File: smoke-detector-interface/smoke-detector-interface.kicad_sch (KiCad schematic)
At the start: 28 parts, among them J1 Conn_01x04_Pin, J2 M50-3500542, J3 DE9_Receptacle, J4 61200621621, J5 Conn_01x06_Pin, U1 UA78L10ACLPRE3, U2 AS7805AT, U3 ATtiny13A-P

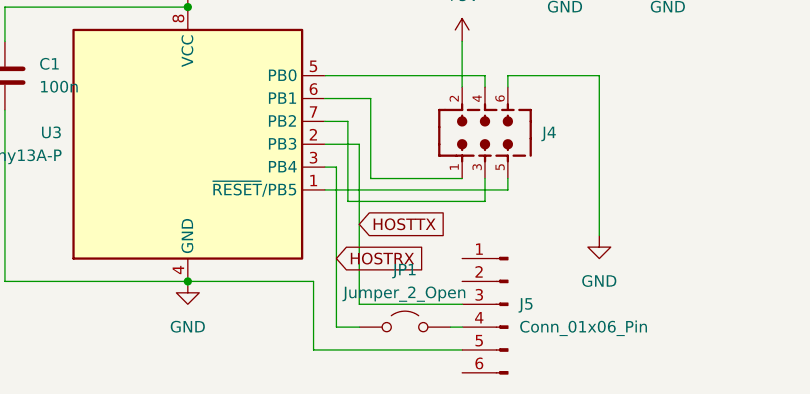
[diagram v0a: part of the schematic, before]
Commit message: WIP
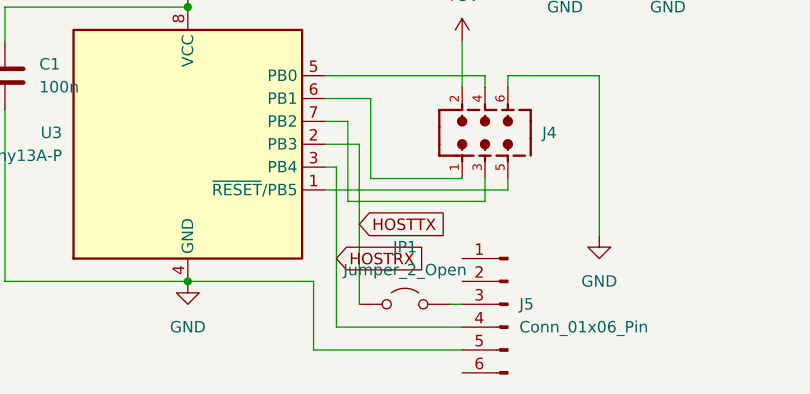
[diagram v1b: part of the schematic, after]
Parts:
- JP1: footprint TestPoint:TestPoint_Bridge_Pitch2.54mm_Drill0.7mm -> Resistor_THT:R_Axial_DIN0204_L3.6mm_D1.6mm_P7.62mm_Horizontal
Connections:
- net HOSTRX: now also J5.4 (Pin_4); no longer JP1.1 (A)
- net HOSTTX: now also JP1.1 (A); no longer J5.3 (Pin_3)
- net at JP1.2 (B): now also J5.3 (Pin_3); no longer J5.4 (Pin_4)
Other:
- moved on the sheet: JP1
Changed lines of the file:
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@@
 	(wire
 		(pts
-			(xy 196.85 143.51) (xy 194.31 143.51)
+			(xy 194.31 143.51) (xy 208.28 143.51)
 		)
 		(stroke
@@
 	(wire
 		(pts
-			(xy 208.28 140.97) (xy 196.85 140.97)
+			(xy 208.28 140.97) (xy 207.01 140.97)
 		)
 		(stroke
@@
 	(wire
 		(pts
-			(xy 208.28 143.51) (xy 207.01 143.51)
-		)
-		(stroke
-			(width 0)
-			(type default)
-		)
-	)
-	(wire
-		(pts
 			(xy 231.14 88.9) (xy 231.14 91.44)
 		)
@@
 	(symbol
 		(lib_id "Jumper:Jumper_2_Open")
-		(at 201.93 143.51 0)
+		(at 201.93 140.97 0)
 		(unit 1)
 		(exclude_from_sim yes)
@@
 		(fields_autoplaced yes)
 		(property "Reference" "JP1"
-			(at 201.93 137.16 0)
+			(at 201.93 134.62 0)
 			(effects
 				(font
@@
 		)
 		(property "Value" "Jumper_2_Open"
-			(at 201.93 139.7 0)
+			(at 201.93 137.16 0)
 			(effects
 				(font
@@
 			)
 		)
-		(property "Footprint" "TestPoint:TestPoint_Bridge_Pitch2.54mm_Drill0.7mm"
-			(at 201.93 143.51 0)
+		(property "Footprint" "Resistor_THT:R_Axial_DIN0204_L3.6mm_D1.6mm_P7.62mm_Horizontal"
+			(at 201.93 140.97 0)
 			(effects
 				(font
@@
 		)
 		(property "Datasheet" "~"
-			(at 201.93 143.51 0)
+			(at 201.93 140.97 0)
 			(effects
 				(font
@@
 		)
 		(property "Description" "Jumper, 2-pole, open"
-			(at 201.93 143.51 0)
+			(at 201.93 140.97 0)
 			(effects
 				(font

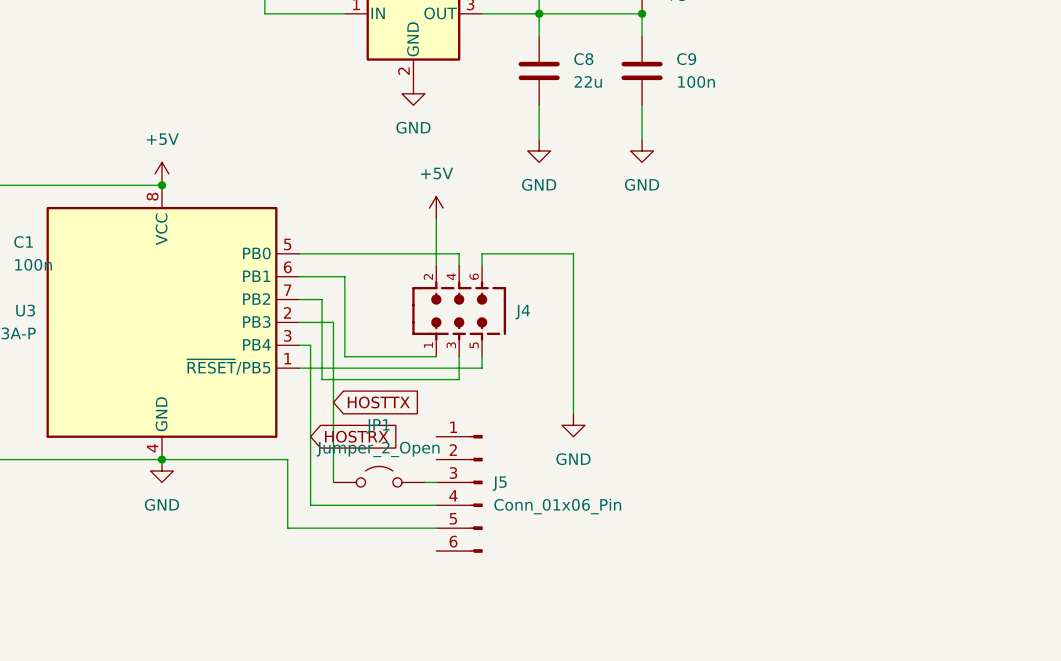
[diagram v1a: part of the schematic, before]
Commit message: Improved routing.
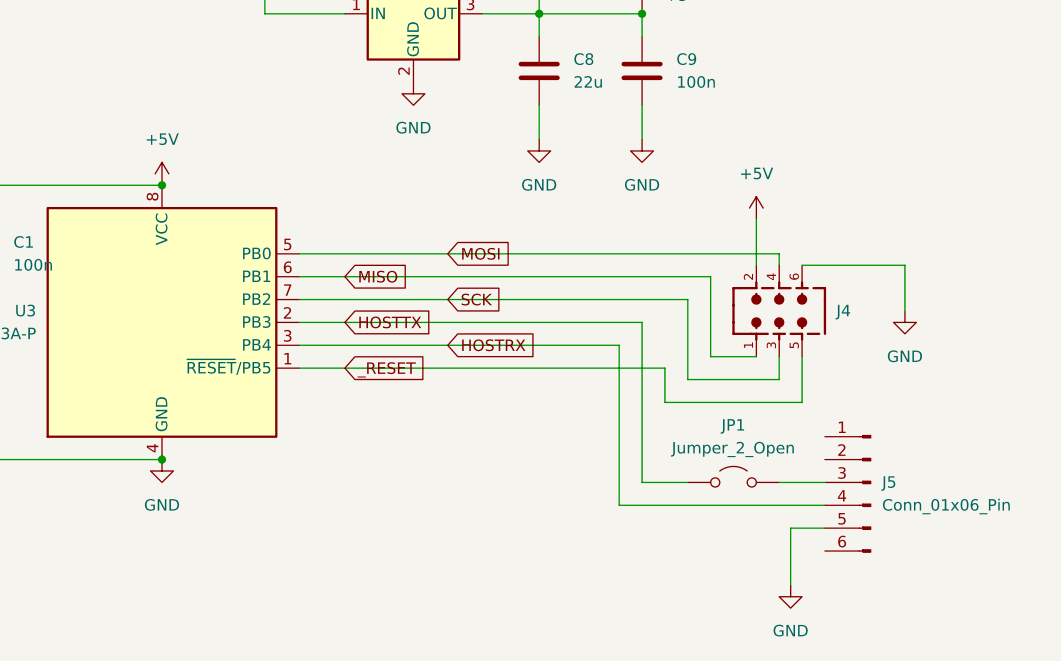
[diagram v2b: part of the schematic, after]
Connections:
- net _RESET: now also J4.5, U3.1 (~{RESET}/PB5)
- net MOSI: now reaches J4.4, U3.5 (PB0)
- net MISO: now reaches J4.1, U3.6 (PB1)
- net SCK: now reaches J4.3, U3.7 (PB2)
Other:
- moved on the sheet: J4, J5, JP1
